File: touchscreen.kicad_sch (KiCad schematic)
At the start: 5 parts, among them U3 CST816D, U4 GC9A01_TFT, U5 TXS0108EPWR

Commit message: reste routage mais peu
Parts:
- U3: footprint MyGlove:PinHeader_1x04_Pas2.54mm -> MyGlove:PinHeader_1x04_P2.54mm_Vertical
- U4: footprint MyGlove:PinHeader_1x08_Pas2.54mm -> MyGlove:PinHeader_1x08_P2.54mm_Vertical
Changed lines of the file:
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@@
 			)
 		)
-		(property "Footprint" "MyGlove:PinHeader_1x04_Pas2.54mm"
+		(property "Footprint" "MyGlove:PinHeader_1x04_P2.54mm_Vertical"
 			(at 91.44 119.38 0)
 			(hide yes)
@@
 			)
 		)
-		(property "Footprint" "MyGlove:PinHeader_1x08_Pas2.54mm"
+		(property "Footprint" "MyGlove:PinHeader_1x08_P2.54mm_Vertical"
 			(at 93.98 64.77 0)
 			(hide yes)

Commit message: Regles de design
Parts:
- D3: footprint MyGlove:LED -> MyGlove:D_0603_1608Metric_Pad1.05x0.95mm_HandSolder
- U3: footprint MyGlove:PinHeader_1x04_P2.54mm_Vertical -> MyGlove:PinHeader_1x04_Pas2.54mm_cst816d
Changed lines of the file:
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@@
 			)
 		)
-		(property "Footprint" "MyGlove:PinHeader_1x04_P2.54mm_Vertical"
+		(property "Footprint" "MyGlove:PinHeader_1x04_Pas2.54mm_cst816d"
 			(at 91.44 119.38 0)
 			(hide yes)
@@
 			)
 		)
-		(property "Footprint" "MyGlove:LED"
+		(property "Footprint" "MyGlove:D_0603_1608Metric_Pad1.05x0.95mm_HandSolder"
 			(at 104.14 40.64 0)
 			(hide yes)

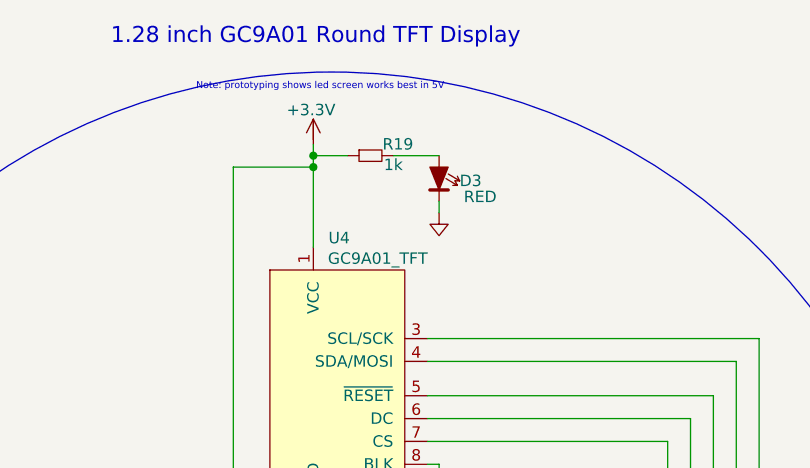
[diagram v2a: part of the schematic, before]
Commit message: Debut potable
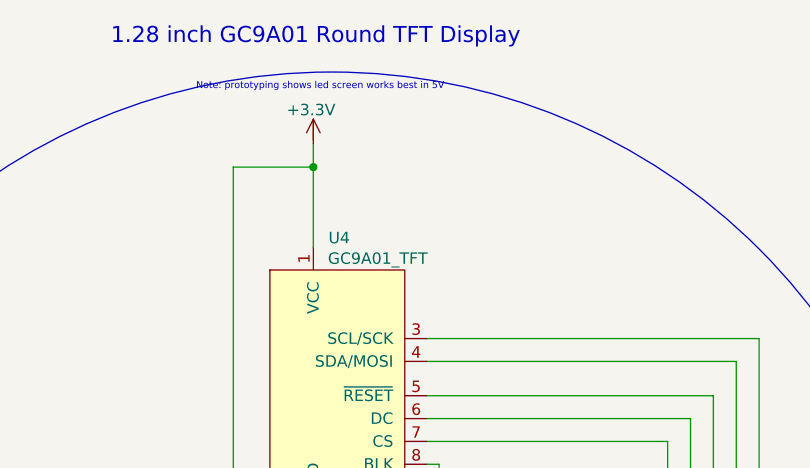
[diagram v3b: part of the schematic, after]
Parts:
- removed D3: RED, MyGlove:D_0603_1608Metric_Pad1.05x0.95mm_HandSolder, symbol G-Love:LED_Indicator
- removed R19: 1k, MyGlove:Resistor_0603, symbol G-Love:R

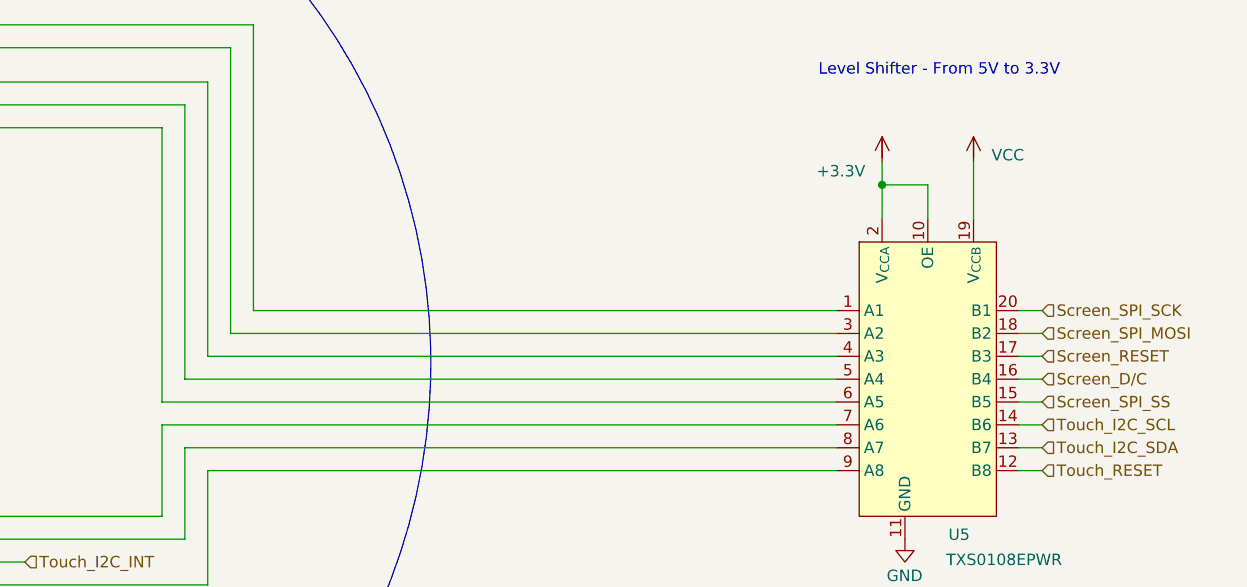
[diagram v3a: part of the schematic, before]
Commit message: Passe ERC
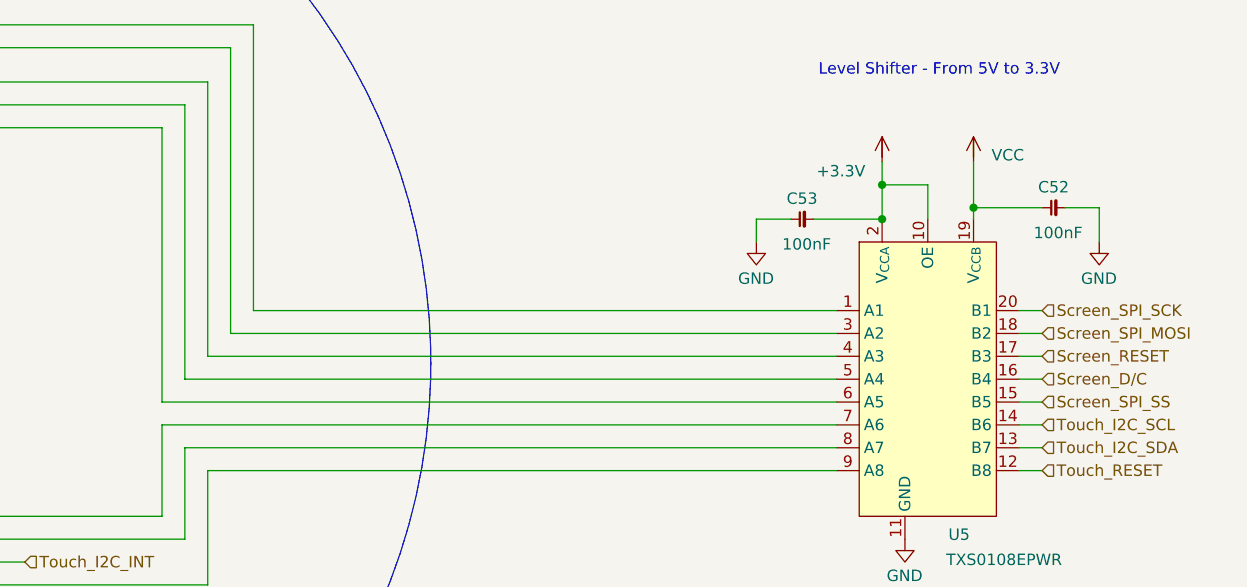
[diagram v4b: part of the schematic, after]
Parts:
- added C52, C53: 100nF, MyGlove:Capacitor_0603, symbol G-Love:C
- U3: footprint MyGlove:PinHeader_1x04_Pas2.54mm_cst816d -> MyGlove:PinHeader_1x04_P2.54mm_Vertical_CST816D
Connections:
- net +3.3V: now also C53.1
- net GND: now also C52.1, C53.2
- net VCC: now also C52.2
